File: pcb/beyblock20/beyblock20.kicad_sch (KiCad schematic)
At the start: 45 parts, among them J1 Conn_01x04_Female, J2 Conn_01x04_Male, SW1 SW_SPST, SW10 SW_SPST, SW11 SW_SPST, SW12 SW_SPST, SW13 SW_SPST, SW14 SW_SPST, SW15 SW_SPST, SW16 SW_SPST, SW17 SW_SPST, SW18 SW_SPST, SW19 SW_SPST, SW2 SW_SPST, SW20 SW_SPST, SW3 SW_SPST, SW4 SW_SPST, SW5 SW_SPST, SW6 SW_SPST, SW7 SW_SPST, SW8 SW_SPST, SW9 SW_SPST, U1 SeeeduinoXIAO

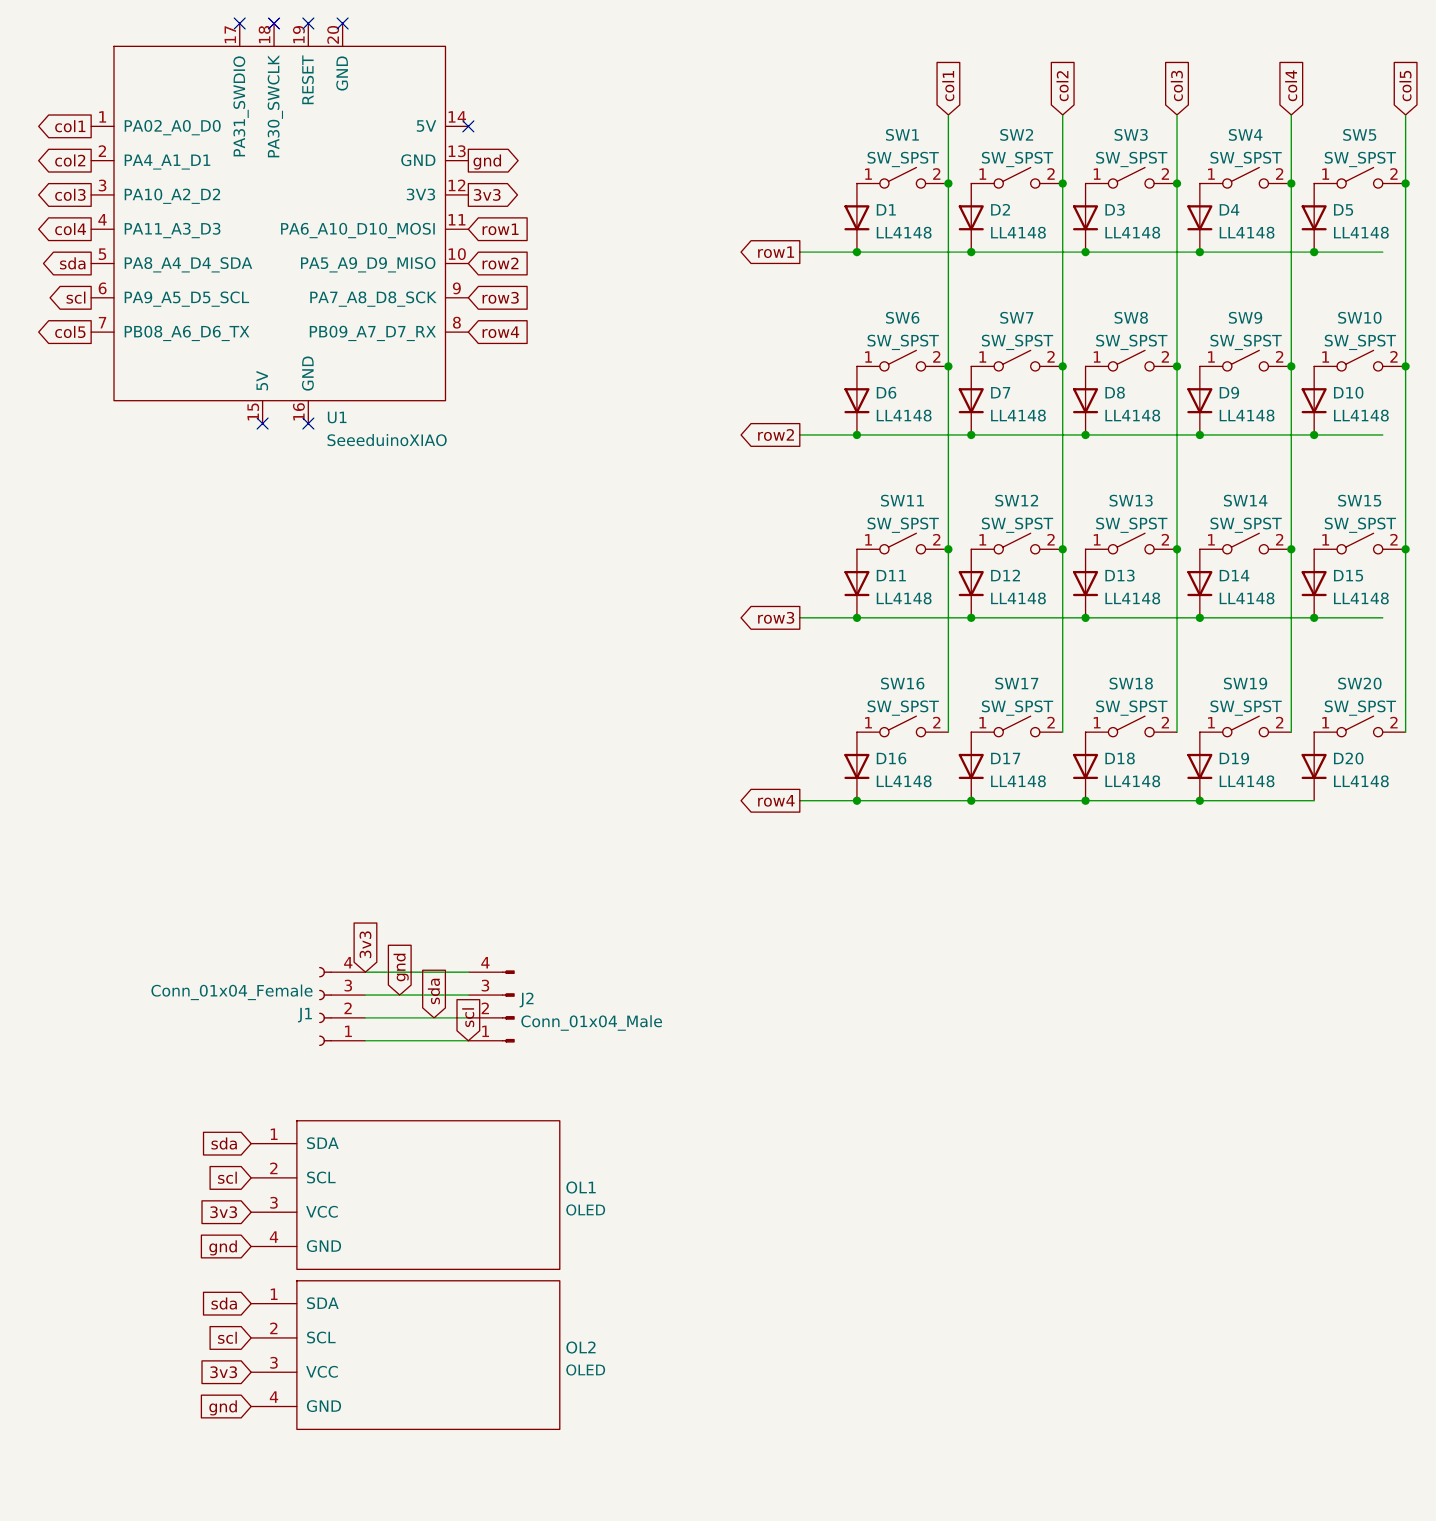
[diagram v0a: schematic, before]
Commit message: finish initial pcb
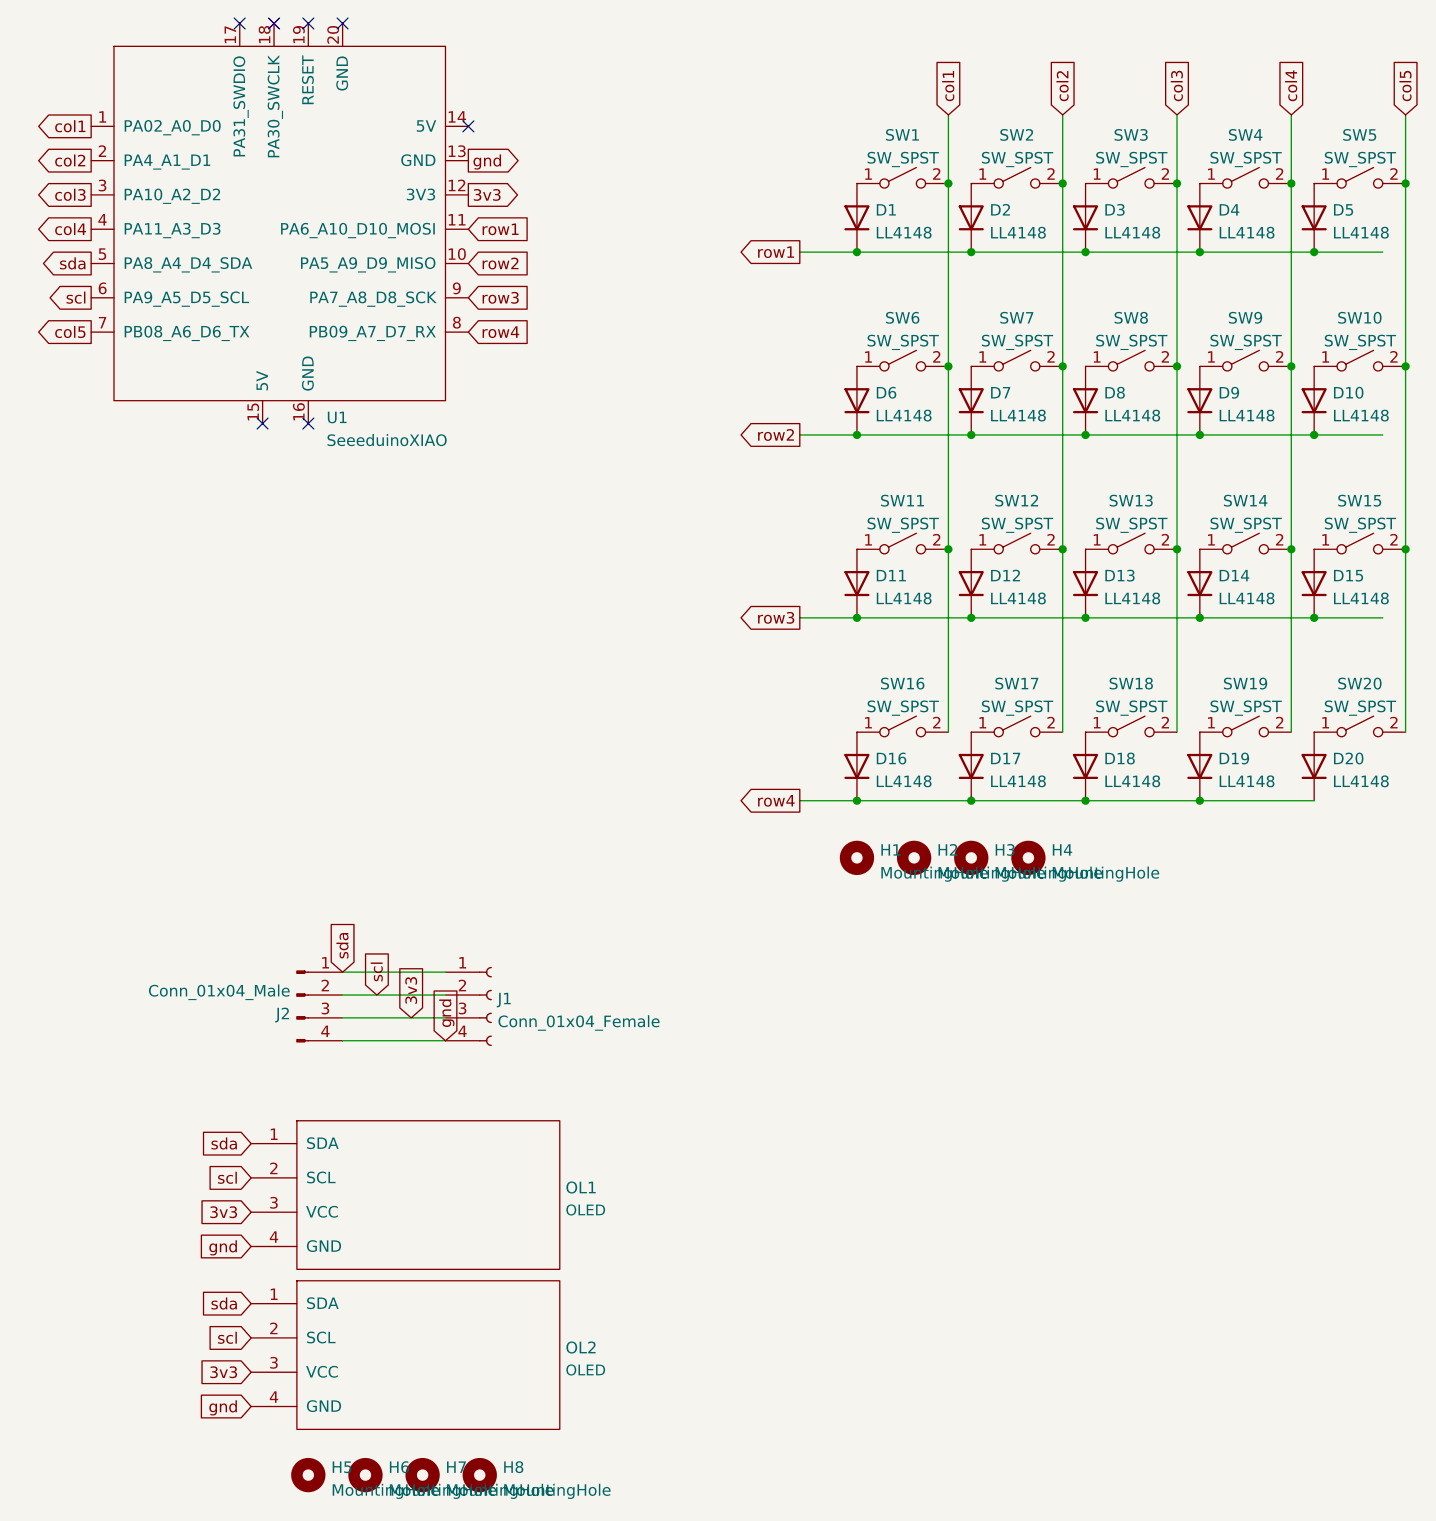
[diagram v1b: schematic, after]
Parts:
- added H1, H2, H3, H4, H5, H6, H7, H8: MountingHole, symbol Mechanical:MountingHole
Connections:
- net 3v3: now also J1.3 (Pin_3), J2.3 (Pin_3); no longer J1.4 (Pin_4), J2.4 (Pin_4)
- net gnd: now also J1.4 (Pin_4), J2.4 (Pin_4); no longer J1.3 (Pin_3), J2.3 (Pin_3)
- net scl: now also J1.2 (Pin_2), J2.2 (Pin_2); no longer J1.1 (Pin_1), J2.1 (Pin_1)
- net sda: now also J1.1 (Pin_1), J2.1 (Pin_1); no longer J1.2 (Pin_2), J2.2 (Pin_2)
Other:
- moved on the sheet: J1, J2

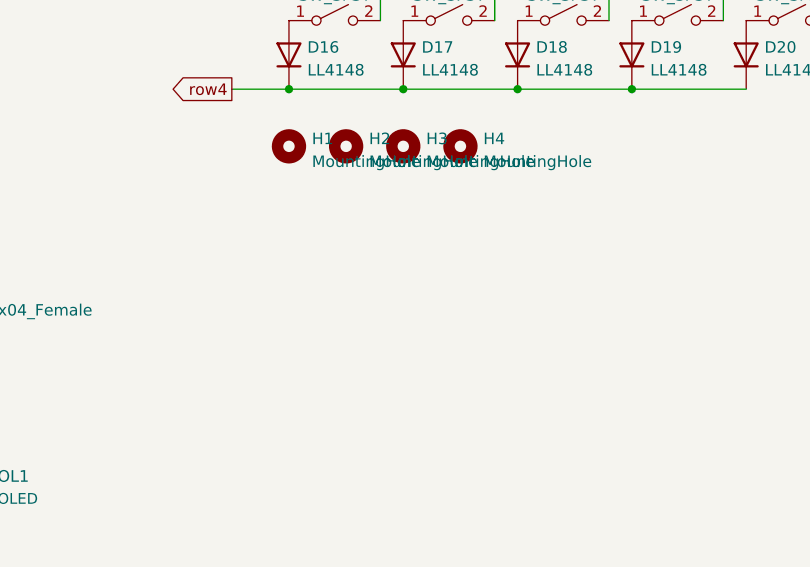
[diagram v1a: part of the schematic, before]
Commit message: add trrs
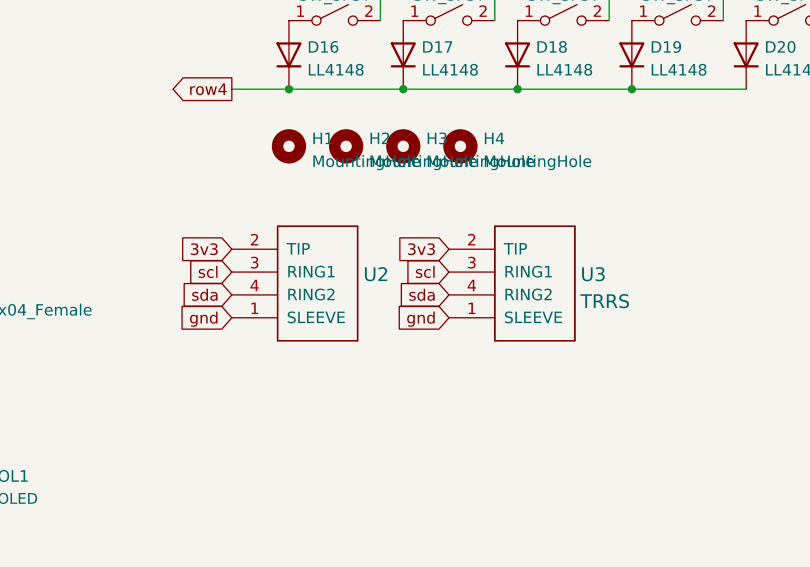
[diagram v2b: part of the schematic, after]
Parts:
- added U2: (no value), symbol keebio:TRRS
- added U3: TRRS, symbol keebio:TRRS
- H1, H2, H3, H4, H5, H6, H7, H8: footprint (none) -> MountingHole:MountingHole_2.2mm_M2
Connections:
- net 3v3: now also U2.2 (TIP), U3.2 (TIP)
- net gnd: now also U2.1 (SLEEVE), U3.1 (SLEEVE)
- net scl: now also U2.3 (RING1), U3.3 (RING1)
- net sda: now also U2.4 (RING2), U3.4 (RING2)
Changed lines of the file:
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@@
+    )
+  )
+  (global_label "scl" (shape input) (at 133.35 128.27 180) (fields_autoplaced)
+    (effects (font (size 1.27 1.27)) (justify right))
+    (property "Intersheet References" "${INTERSHEET_REFS}" (id 0) (at 128.155 128.1906 0)
+      (effects (font (size 1.27 1.27)) (justify right) hide)
     )
   )
@@
     )
   )
+  (global_label "sda" (shape input) (at 109.22 130.81 180) (fields_autoplaced)
+    (effects (font (size 1.27 1.27)) (justify right))
+    (property "Intersheet References" "${INTERSHEET_REFS}" (id 0) (at 103.4807 130.7306 0)
+      (effects (font (size 1.27 1.27)) (justify right) hide)
+    )
+  )
   (global_label "gnd" (shape input) (at 48.26 175.26 180) (fields_autoplaced)
     (effects (font (size 1.27 1.27)) (justify right))
@@
     )
   )
+  (global_label "sda" (shape input) (at 133.35 130.81 180) (fields_autoplaced)
+    (effects (font (size 1.27 1.27)) (justify right))
+    (property "Intersheet References" "${INTERSHEET_REFS}" (id 0) (at 127.6107 130.7306 0)
+      (effects (font (size 1.27 1.27)) (justify right) hide)
+    )
+  )
+  (global_label "3v3" (shape input) (at 109.22 125.73 180) (fields_autoplaced)
+    (effects (font (size 1.27 1.27)) (justify right))
+    (property "Intersheet References" "${INTERSHEET_REFS}" (id 0) (at 103.4202 125.6506 0)
+      (effects (font (size 1.27 1.27)) (justify right) hide)
+    )
+  )
+  (global_label "scl" (shape input) (at 109.22 128.27 180) (fields_autoplaced)
+    (effects (font (size 1.27 1.27)) (justify right))
+    (property "Intersheet References" "${INTERSHEET_REFS}" (id 0) (at 104.025 128.1906 0)
+      (effects (font (size 1.27 1.27)) (justify right) hide)
+    )
+  )
   (global_label "row4" (shape output) (at 109.22 107.95 180) (fields_autoplaced)
     (effects (font (size 1.27 1.27)) (justify right))
@@
     (effects (font (size 1.27 1.27)) (justify right))
     (property "Intersheet References" "${INTERSHEET_REFS}" (id 0) (at 23.9545 40.5606 0)
+      (effects (font (size 1.27 1.27)) (justify right) hide)
+    )
+  )
+  (global_label "3v3" (shape input) (at 133.35 125.73 180) (fields_autoplaced)
+    (effects (font (size 1.27 1.27)) (justify right))
+    (property "Intersheet References" "${INTERSHEET_REFS}" (id 0) (at 127.5502 125.6506 0)
       (effects (font (size 1.27 1.27)) (justify right) hide)
     )
@@
     )
   )
+  (global_label "gnd" (shape input) (at 133.35 133.35 180) (fields_autoplaced)
+    (effects (font (size 1.27 1.27)) (justify right))
+    (property "Intersheet References" "${INTERSHEET_REFS}" (id 0) (at 127.4898 133.2706 0)
+      (effects (font (size 1.27 1.27)) (justify right) hide)
+    )
+  )
   (global_label "row3" (shape input) (at 72.39 52.07 0) (fields_autoplaced)
     (effects (font (size 1.27 1.27)) (justify left))
@@
     )
   )
+  (global_label "gnd" (shape input) (at 109.22 133.35 180) (fields_autoplaced)
+    (effects (font (size 1.27 1.27)) (justify right))
+    (property "Intersheet References" "${INTERSHEET_REFS}" (id 0) (at 103.3598 133.2706 0)
+      (effects (font (size 1.27 1.27)) (justify right) hide)
+    )
+  )
   (global_label "scl" (shape input) (at 48.26 167.64 180) (fields_autoplaced)
     (effects (font (size 1.27 1.27)) (justify right))
@@
     (pin "2")
   )
+  (symbol (lib_id "keebio:TRRS") (at 118.11 135.89 0) (unit 1)
+    (in_bom yes) (on_board yes) (fields_autoplaced)
+    (property "Reference" "U2" (id 0) (at 123.825 128.5638 0)
+      (effects (font (size 1.524 1.524)) (justify left))
+    )
+    (property "Value" "" (id 1) (at 123.825 131.5572 0)
+      (effects (font (size 1.524 1.524)) (justify left))
+    )
+    (property "Footprint" "" (id 2) (at 121.92 135.89 0)
+      (effects (font (size 1.524 1.524)) hide)
+    )
+    (property "Datasheet" "" (id 3) (at 121.92 135.89 0)
+      (effects (font (size 1.524 1.524)) hide)
+    )
+    (pin "1")
+    (pin "2")
+    (pin "3")
+    (pin "4")
+  )
   (symbol (lib_id "Diode:LL4148") (at 115.57 63.5 90) (unit 1)
     (in_bom yes) (on_board yes) (fields_autoplaced)
@@
       (effects (font (size 1.27 1.27)) (justify left))
     )
-    (property "Footprint" "" (id 2) (at 115.57 114.3 0)
+    (property "Footprint" "MountingHole:MountingHole_2.2mm_M2" (id 2) (at 115.57 114.3 0)
       (effects (font (size 1.27 1.27)) hide)
     )
@@
     (pin "2")
   )
+  (symbol (lib_id "keebio:TRRS") (at 142.24 135.89 0) (unit 1)
+    (in_bom yes) (on_board yes) (fields_autoplaced)
+    (property "Reference" "U3" (id 0) (at 147.955 128.5638 0)
+      (effects (font (size 1.524 1.524)) (justify left))
+    )
+    (property "Value" "TRRS" (id 1) (at 147.955 131.5572 0)
+      (effects (font (size 1.524 1.524)) (justify left))
+    )
+    (property "Footprint" "" (id 2) (at 146.05 135.89 0)
+      (effects (font (size 1.524 1.524)) hide)
+    )
+    (property "Datasheet" "" (id 3) (at 146.05 135.89 0)
+      (effects (font (size 1.524 1.524)) hide)
+    )
+    (pin "1")
+    (pin "2")
+    (pin "3")
+    (pin "4")
+  )
   (symbol (lib_id "Switch:SW_SPST") (at 133.35 80.01 0) (unit 1)
     (in_bom yes) (on_board yes) (fields_autoplaced)
@@
       (effects (font (size 1.27 1.27)) (justify left))
     )
-    (property "Footprint" "" (id 2) (at 60.96 182.88 0)
+    (property "Footprint" "MountingHole:MountingHole_2.2mm_M2" (id 2) (at 60.96 182.88 0)
       (effects (font (size 1.27 1.27)) hide)
     )
@@
       (effects (font (size 1.27 1.27)) (justify left))
     )
-    (property "Footprint" "" (id 2) (at 121.92 114.3 0)
+    (property "Footprint" "MountingHole:MountingHole_2.2mm_M2" (id 2) (at 121.92 114.3 0)
       (effects (font (size 1.27 1.27)) hide)
     )
@@
       (effects (font (size 1.27 1.27)) (justify left))
     )
-    (property "Footprint" "" (id 2) (at 134.62 114.3 0)
+    (property "Footprint" "MountingHole:MountingHole_2.2mm_M2" (id 2) (at 134.62 114.3 0)
       (effects (font (size 1.27 1.27)) hide)
     )
@@
       (effects (font (size 1.27 1.27)) (justify left))
     )
-    (property "Footprint" "" (id 2) (at 67.31 182.88 0)
+    (property "Footprint" "MountingHole:MountingHole_2.2mm_M2" (id 2) (at 67.31 182.88 0)
       (effects (font (size 1.27 1.27)) hide)
     )
@@
       (effects (font (size 1.27 1.27)) (justify left))
     )
-    (property "Footprint" "" (id 2) (at 54.61 182.88 0)
+    (property "Footprint" "MountingHole:MountingHole_2.2mm_M2" (id 2) (at 54.61 182.88 0)
       (effects (font (size 1.27 1.27)) hide)
     )
@@
       (effects (font (size 1.27 1.27)) (justify left))
     )
-    (property "Footprint" "" (id 2) (at 128.27 114.3 0)
+    (property "Footprint" "MountingHole:MountingHole_2.2mm_M2" (id 2) (at 128.27 114.3 0)
       (effects (font (size 1.27 1.27)) hide)
     )
@@
       (effects (font (size 1.27 1.27)) (justify left))
     )
-    (property "Footprint" "" (id 2) (at 73.66 182.88 0)
+    (property "Footprint" "MountingHole:MountingHole_2.2mm_M2" (id 2) (at 73.66 182.88 0)
       (effects (font (size 1.27 1.27)) hide)
     )
@@
       (reference "U1") (unit 1) (value "SeeeduinoXIAO") (footprint "Seeeduino XIAO KICAD:Seeeduino XIAO-MOUDLE14P-2.54-21X17.8MM")
     )
-  )
+    (path "/1440444c-7b3c-4048-bee5-f38a07cb6ccb"
+      (reference "U2") (unit 1) (value "TRRS") (footprint "Keebio-Parts:TRRS-PJ-320A")
+    )
+    (path "/5c2f63e8-3854-47c2-b529-57fcc99ef42d"
+      (reference "U3") (unit 1) (value "TRRS") (footprint "Keebio-Parts:TRRS-PJ-320A")
+    )
+  )
